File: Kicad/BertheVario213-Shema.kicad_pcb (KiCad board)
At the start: 2 copper layers, 42 x 96.5 mm, 16 parts, among them Q1 S8050, SW1 gauche, SW2 centre, SW3 droite

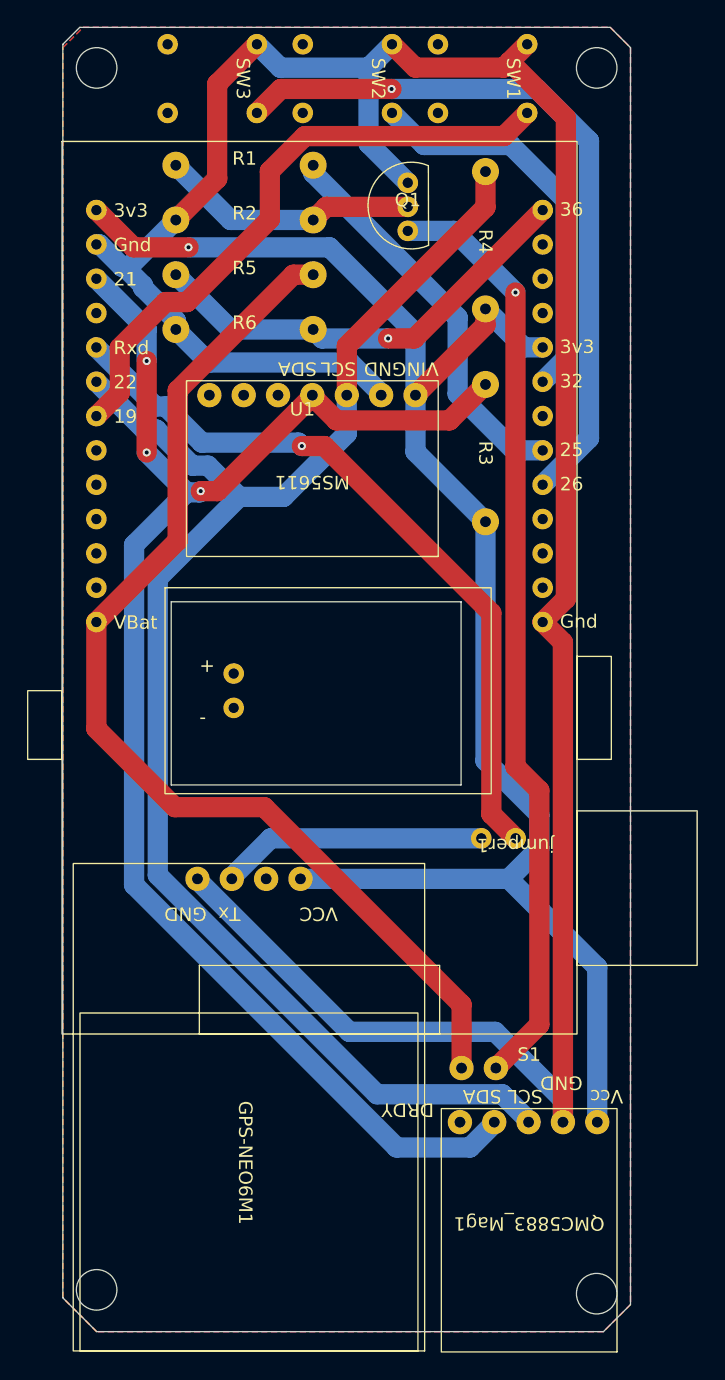
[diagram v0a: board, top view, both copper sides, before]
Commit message: modif pcb
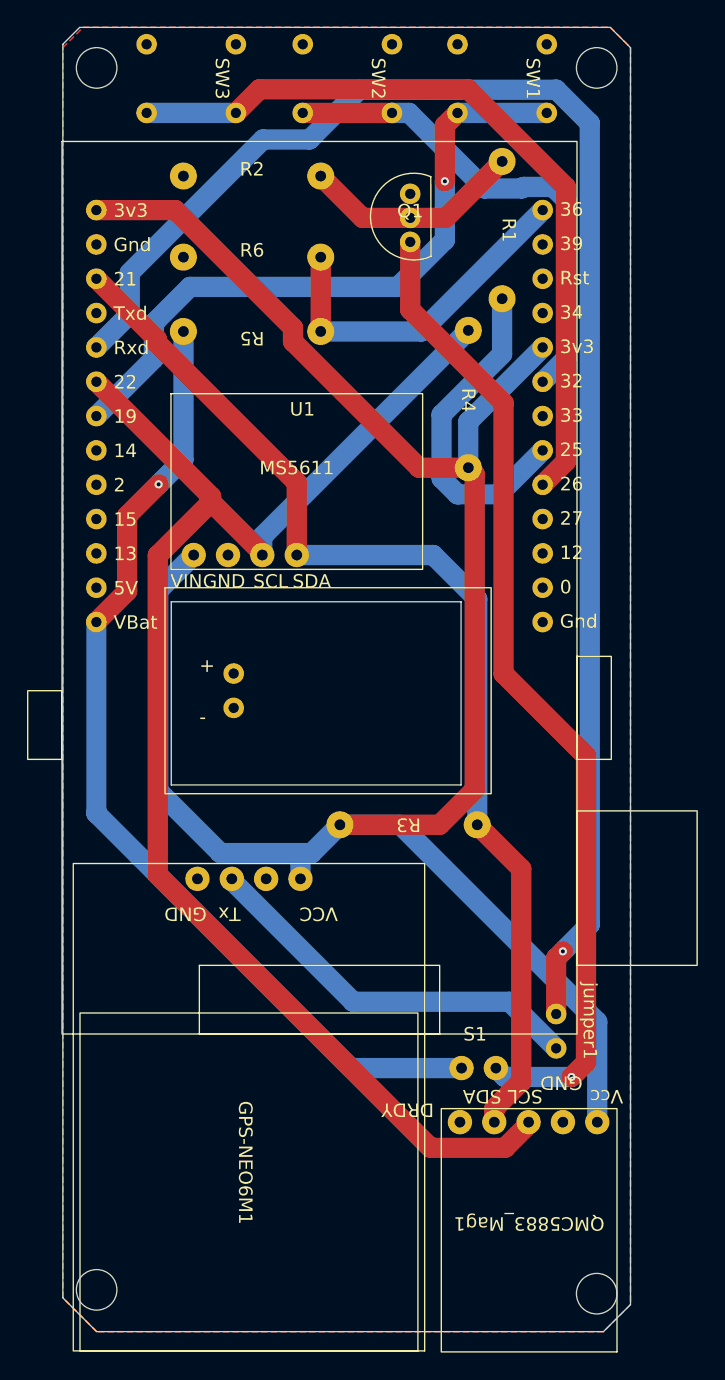
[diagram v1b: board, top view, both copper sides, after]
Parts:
- moved R3 28.1 mm to (147.1, 120.0), turned to 180 degrees
- moved R1 19.7 mm to (154.0, 76.0), turned to -90 degrees
- moved jumper1 13.3 mm to (158.0, 134.0), turned to -90 degrees
- moved R4 11.8 mm to (151.5, 88.5)
- moved MS5611 11.1 mm to (135.0, 97.5), turned to 0 degrees
- moved R6 5.38 mm to (135.5, 78.0)
- moved R5 4.24 mm to (135.5, 83.5), turned to 180 degrees
- moved R2 3.30 mm to (135.5, 72.0)
- moved SW3 1.55 mm to (132.8, 64.8)
- moved SW1 1.45 mm to (155.8, 64.8)
- moved Q1 0.84 mm to (147.2, 75.1)
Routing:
- net GNDREF: track 196.5 -> 0.00 mm
- net Net-(U1-Rxd): track 54.8 -> 114.2 mm
- net Net-(MS5611-SDA): track 111.7 -> 82.2 mm, vias 3 -> 0
- net Net-(GPS-NEO6M1-VCC): track 122.5 -> 151.4 mm, vias 1 -> 0
- net Net-(GPS-NEO6M1-TX): track 19.8 -> 29.3 mm
- net Net-(U1-Vbat): track 81.3 -> 73.1 mm, vias 0 -> 1
- net Net-(U1-In_Vbat): track 33.0 -> 25.6 mm, vias 1 -> 0
- net Net-(U1-Bouton_Centre): track 29.7 -> 36.4 mm
- net Net-(MS5611-SCL): track 113.2 -> 106.7 mm
- net Net-(U1-Speaker): track 29.4 -> 24.5 mm
- net Net-(Q1-C): track 69.3 -> 73.5 mm
- net Net-(U1-Bouton_Gauche): track 45.2 -> 49.1 mm, vias 0 -> 1
- net Net-(U1-Bouton_Droit): track 53.8 -> 57.5 mm, vias 1 -> 0
- net Net-(Q1-B): track 19.2 -> 16.4 mm
